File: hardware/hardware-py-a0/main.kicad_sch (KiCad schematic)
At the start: 58 parts, among them J6 USB_C_Receptacle_USB2.0_16P, J7 Conn_02x08_Odd_Even, Q6 BSS138, SW1 SW_Push, SW10 SW_Push, SW11 SW_Push, SW12 SW_Push, SW13 SW_Push, SW14 SW_Push, SW15 SW_Push, SW16 SW_Push, SW17 SW_Push, SW18 SW_Push, SW19 SW_Push, SW2 SW_Push, SW20 SW_Push, SW21 Encoder, SW22 SW_Push, SW3 SW_Push, SW4 SW_Push, SW5 SW_Push, SW6 SW_Push, SW7 SW_Push, SW8 SW_Push, SW9 SW_Push, U3 74HC595, U4 ESP32-S3-WROOM-1

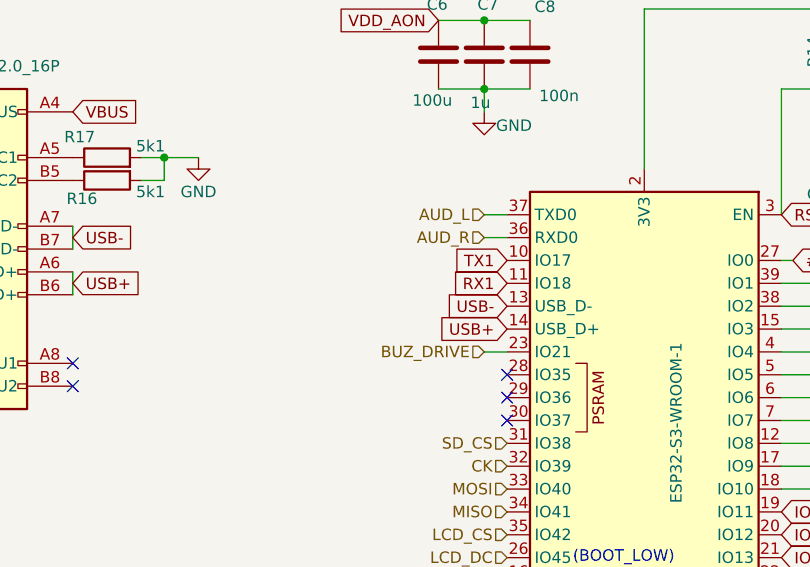
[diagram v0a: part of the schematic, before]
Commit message: hw: power management begin
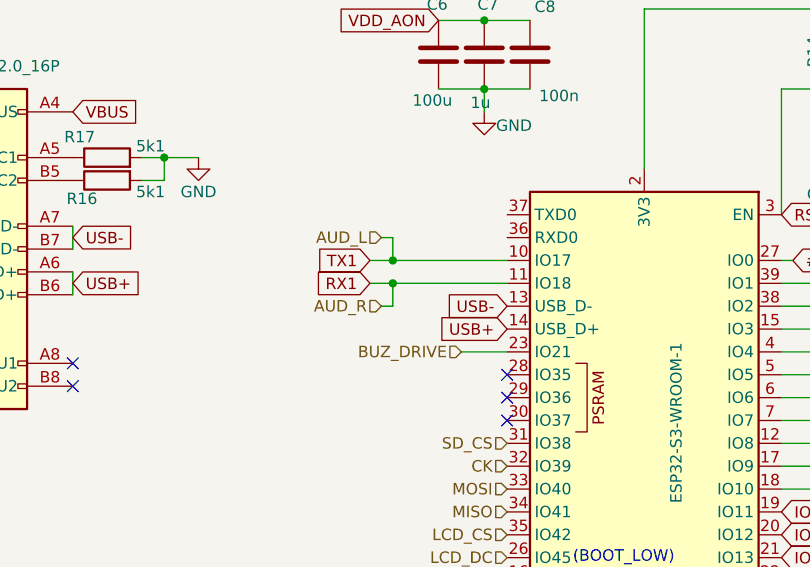
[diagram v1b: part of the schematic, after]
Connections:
- net AUD_L: no longer names the net of U4.37 (TXD0)
- net AUD_R: no longer names the net of U4.36 (RXD0)
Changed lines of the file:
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@@
+	)
+	(junction
+		(at 96.52 124.46)
+		(diameter 0)
+		(color 0 0 0 0)
 	)
 	(junction
@@
 	(junction
 		(at 190.5 60.96)
+		(diameter 0)
+		(color 0 0 0 0)
+	)
+	(junction
+		(at 96.52 127)
 		(diameter 0)
 		(color 0 0 0 0)
@@
 	(wire
 		(pts
-			(xy 109.22 119.38) (xy 106.68 119.38)
+			(xy 93.98 127) (xy 96.52 127)
 		)
 		(stroke
@@
 	(wire
 		(pts
+			(xy 95.25 121.92) (xy 96.52 121.92)
+		)
+		(stroke
+			(width 0)
+			(type default)
+		)
+	)
+	(wire
+		(pts
 			(xy 172.72 54.61) (xy 193.04 54.61)
 		)
@@
 	(wire
 		(pts
+			(xy 95.25 129.54) (xy 96.52 129.54)
+		)
+		(stroke
+			(width 0)
+			(type default)
+		)
+	)
+	(wire
+		(pts
 			(xy 139.7 144.78) (xy 157.48 144.78)
 		)
@@
 	(wire
 		(pts
+			(xy 96.52 127) (xy 109.22 127)
+		)
+		(stroke
+			(width 0)
+			(type default)
+		)
+	)
+	(wire
+		(pts
 			(xy 129.54 60.96) (xy 129.54 71.12)
 		)
@@
 	(wire
 		(pts
+			(xy 96.52 121.92) (xy 96.52 124.46)
+		)
+		(stroke
+			(width 0)
+			(type default)
+		)
+	)
+	(wire
+		(pts
 			(xy 193.04 60.96) (xy 193.04 64.77)
 		)
@@
 	(wire
 		(pts
-			(xy 109.22 121.92) (xy 106.68 121.92)
-		)
-		(stroke
-			(width 0)
-			(type default)
-		)
-	)
-	(wire
-		(pts
 			(xy 88.9 162.56) (xy 109.22 162.56)
 		)
@@
 	(wire
 		(pts
+			(xy 93.98 124.46) (xy 96.52 124.46)
+		)
+		(stroke
+			(width 0)
+			(type default)
+		)
+	)
+	(wire
+		(pts
 			(xy 152.4 74.93) (xy 152.4 71.12)
 		)
@@
 	(wire
 		(pts
+			(xy 96.52 129.54) (xy 96.52 127)
+		)
+		(stroke
+			(width 0)
+			(type default)
+		)
+	)
+	(wire
+		(pts
 			(xy 152.4 54.61) (xy 152.4 50.8)
 		)
@@
 	(wire
 		(pts
+			(xy 96.52 124.46) (xy 109.22 124.46)
+		)
+		(stroke
+			(width 0)
+			(type default)
+		)
+	)
+	(wire
+		(pts
 			(xy 124.46 96.52) (xy 147.32 96.52)
 		)
@@
 	(wire
 		(pts
-			(xy 106.68 134.62) (xy 109.22 134.62)
+			(xy 104.14 134.62) (xy 109.22 134.62)
 		)
 		(stroke
@@
 	(global_label "TX1"
 		(shape input)
-		(at 109.22 124.46 180)
-		(fields_autoplaced yes)
-		(effects
-			(font
-				(size 1.27 1.27)
-			)
-			(justify right)
-		)
-		(property "Intersheetrefs" "${INTERSHEET_REFS}"
-			(at 102.8482 124.46 0)
+		(at 93.98 124.46 180)
+		(fields_autoplaced yes)
+		(effects
+			(font
+				(size 1.27 1.27)
+			)
+			(justify right)
+		)
+		(property "Intersheetrefs" "${INTERSHEET_REFS}"
+			(at 87.6082 124.46 0)
 			(effects
 				(font
@@
 	(global_label "RX1"
 		(shape input)
-		(at 109.22 127 180)
-		(fields_autoplaced yes)
-		(effects
-			(font
-				(size 1.27 1.27)
-			)
-			(justify right)
-		)
-		(property "Intersheetrefs" "${INTERSHEET_REFS}"
-			(at 102.5458 127 0)
+		(at 93.98 127 180)
+		(fields_autoplaced yes)
+		(effects
+			(font
+				(size 1.27 1.27)
+			)
+			(justify right)
+		)
+		(property "Intersheetrefs" "${INTERSHEET_REFS}"
+			(at 87.3058 127 0)
 			(effects
 				(font
@@
 	(hierarchical_label "AUD_L"
 		(shape input)
-		(at 106.68 119.38 180)
+		(at 95.25 121.92 180)
 		(fields_autoplaced yes)
 		(effects
@@
 	(hierarchical_label "AUD_R"
 		(shape input)
-		(at 106.68 121.92 180)
+		(at 95.25 129.54 180)
 		(fields_autoplaced yes)
 		(effects
@@
 	(hierarchical_label "BUZ_DRIVE"
 		(shape input)
-		(at 106.68 134.62 180)
-		(fields_autoplaced yes)
-		(effects
+		(at 104.14 134.62 180)
+		(fields_autoplaced yes)
+		(effects
